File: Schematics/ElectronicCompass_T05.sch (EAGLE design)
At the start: 60 parts, among them Q1 SPB80P06P, Q2 SPB80P06P, Q3 SPB80P06P, Q4 SPB80P06P, U1 ATMEGA32U4, X1 USBSMD

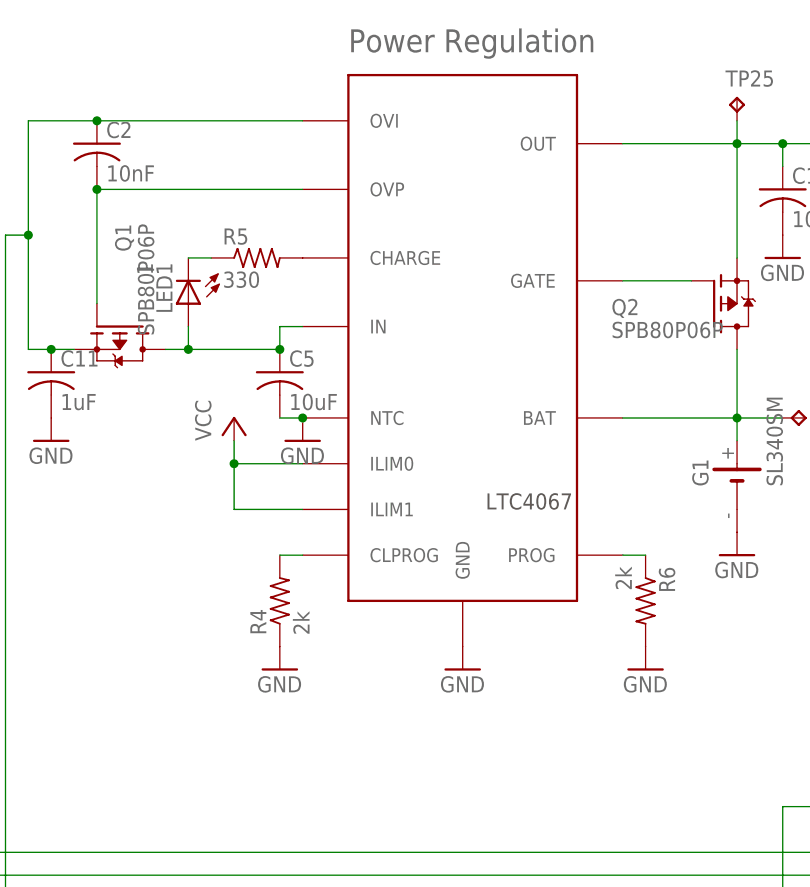
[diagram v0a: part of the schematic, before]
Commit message: board layout continued
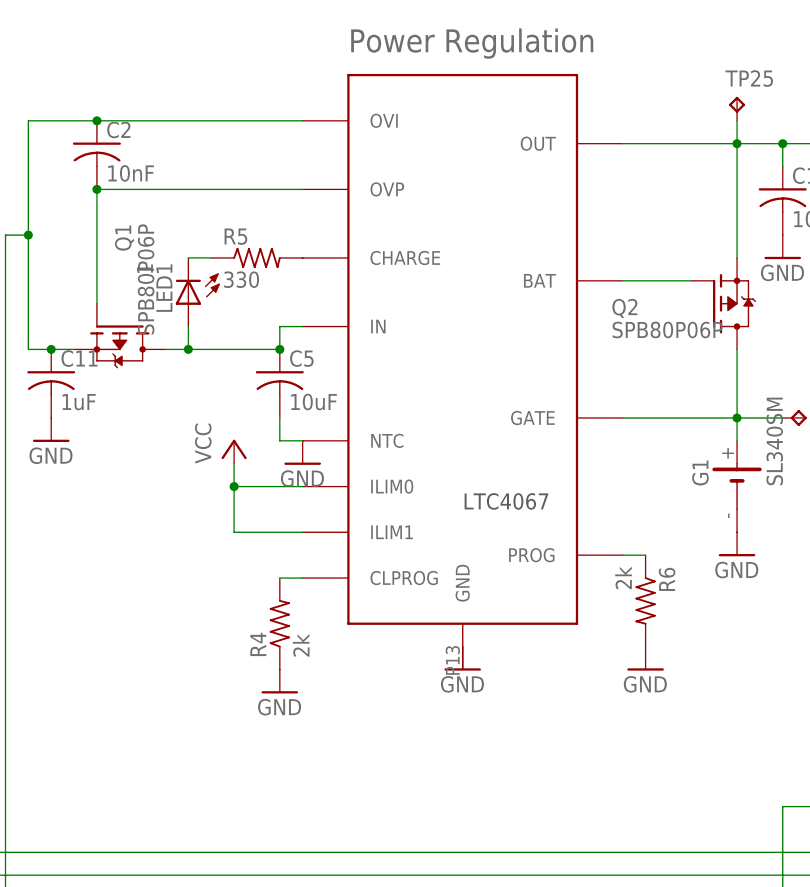
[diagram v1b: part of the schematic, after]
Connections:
- net GND: no longer U$1.GND, U$1.NTC
- net N$16: now also U$1.BAT; no longer U$1.GATE
- net N$4: no longer U$1.CLPROG
- net N$5: now also U$1.GATE; no longer U$1.BAT
- net VCC: no longer U$1.ILIM0, U$1.ILIM1
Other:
- moved on the sheet: R4
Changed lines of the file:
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@@
 <part name="GND14" library="supply1" deviceset="GND" device=""/>
 <part name="C2" library="rcl" deviceset="C-US" device="C0805" value="10nF"/>
-<part name="U$1" library="LTC4067" deviceset="LTC4067" device=""/>
 <part name="C3" library="rcl" deviceset="C-US" device="C0805" value="0.1uF"/>
 <part name="TP26" library="testpad" deviceset="TP" device="TP06R"/>
 <part name="TP27" library="testpad" deviceset="TP" device="TP06R"/>
 <part name="TP28" library="testpad" deviceset="TP" device="TP06R"/>
+<part name="U$1" library="LTC4067" deviceset="LTC4067" device=""/>
 </parts>
 <sheets>
@@
 <frame x1="-25.4" y1="-121.92" x2="276.86" y2="88.9" columns="8" rows="5" layer="97"/>
 <text x="243.84" y="-40.64" size="1.778" layer="97">LCD Mounting/TP</text>
-<text x="53.34" y="27.94" size="1.778" layer="97">LTC4067</text>
+<text x="50.8" y="27.94" size="1.778" layer="97">LTC4067</text>
 <text x="210.82" y="10.16" size="1.778" layer="97">LSM303DLM</text>
 <text x="213.36" y="-66.04" size="1.778" layer="97">Nokia 5110</text>
@@
 <instance part="JP6" gate="G$1" x="175.26" y="-86.36"/>
 <instance part="JP7" gate="G$1" x="182.88" y="-86.36"/>
-<instance part="R4" gate="G$1" x="30.48" y="17.78" rot="R90"/>
+<instance part="R4" gate="G$1" x="30.48" y="15.24" rot="R90"/>
 <instance part="R5" gate="G$1" x="27.94" y="55.88"/>
 <instance part="R6" gate="G$1" x="71.12" y="17.78" rot="R270"/>
@@
 <instance part="GND9" gate="1" x="50.8" y="10.16"/>
 <instance part="GND15" gate="1" x="71.12" y="10.16"/>
-<instance part="GND16" gate="1" x="30.48" y="10.16"/>
-<instance part="P+5" gate="VCC" x="25.4" y="38.1"/>
+<instance part="GND16" gate="1" x="30.48" y="7.62"/>
+<instance part="P+5" gate="VCC" x="25.4" y="35.56"/>
 <instance part="LED1" gate="G$1" x="20.32" y="50.8" rot="R180"/>
 <instance part="Q1" gate="G$1" x="12.7" y="48.26" rot="MR270"/>
@@
 <instance part="C12" gate="G$1" x="76.2" y="-17.78"/>
 <instance part="GND17" gate="1" x="76.2" y="-25.4"/>
-<instance part="GND18" gate="1" x="33.02" y="35.56"/>
+<instance part="GND18" gate="1" x="33.02" y="33.02"/>
 <instance part="G1" gate="G$1" x="81.28" y="30.48" rot="R90"/>
 <instance part="GND19" gate="1" x="81.28" y="22.86"/>
@@
 <instance part="GND14" gate="1" x="5.08" y="35.56"/>
 <instance part="C2" gate="G$1" x="10.16" y="68.58"/>
-<instance part="U$1" gate="G$1" x="50.8" y="40.64" rot="R270"/>
 <instance part="C3" gate="G$1" x="121.92" y="7.62"/>
 <instance part="TP26" gate="G$1" x="180.34" y="-33.02" rot="R270"/>
 <instance part="TP27" gate="G$1" x="180.34" y="-48.26" rot="R270"/>
 <instance part="TP28" gate="G$1" x="180.34" y="-43.18" rot="R270"/>
+<instance part="U$1" gate="G$1" x="50.8" y="45.72" rot="R270"/>
 </instances>
 <busses>
@@
 <pinref part="GND18" gate="1" pin="GND"/>
 <pinref part="C5" gate="G$1" pin="2"/>
-<wire x1="30.48" y1="38.1" x2="33.02" y2="38.1" width="0.1524" layer="91"/>
-<pinref part="U$1" gate="G$1" pin="NTC"/>
-<junction x="33.02" y="38.1"/>
+<wire x1="30.48" y1="38.1" x2="30.48" y2="35.56" width="0.1524" layer="91"/>
+<wire x1="30.48" y1="35.56" x2="33.02" y2="35.56" width="0.1524" layer="91"/>
 </segment>
 <segment>
 <pinref part="C11" gate="G$1" pin="2"/>
 <pinref part="GND14" gate="1" pin="GND"/>
-</segment>
-<segment>
-<pinref part="GND9" gate="1" pin="GND"/>
-<pinref part="U$1" gate="G$1" pin="GND"/>
 </segment>
 <segment>
@@
 </segment>
 <segment>
-<wire x1="33.02" y1="27.94" x2="25.4" y2="27.94" width="0.1524" layer="91"/>
+<wire x1="33.02" y1="25.4" x2="25.4" y2="25.4" width="0.1524" layer="91"/>
 <pinref part="P+5" gate="VCC" pin="VCC"/>
-<wire x1="25.4" y1="27.94" x2="25.4" y2="33.02" width="0.1524" layer="91"/>
-<wire x1="25.4" y1="33.02" x2="25.4" y2="35.56" width="0.1524" layer="91"/>
-<wire x1="33.02" y1="33.02" x2="25.4" y2="33.02" width="0.1524" layer="91"/>
-<junction x="25.4" y="33.02"/>
-<pinref part="U$1" gate="G$1" pin="ILIM0"/>
-<pinref part="U$1" gate="G$1" pin="ILIM1"/>
+<wire x1="25.4" y1="25.4" x2="25.4" y2="30.48" width="0.1524" layer="91"/>
+<wire x1="25.4" y1="30.48" x2="25.4" y2="33.02" width="0.1524" layer="91"/>
+<wire x1="33.02" y1="30.48" x2="25.4" y2="30.48" width="0.1524" layer="91"/>
+<junction x="25.4" y="30.48"/>
 </segment>
 </net>
@@
 <segment>
 <pinref part="R4" gate="G$1" pin="2"/>
-<wire x1="30.48" y1="22.86" x2="33.02" y2="22.86" width="0.1524" layer="91"/>
-<pinref part="U$1" gate="G$1" pin="CLPROG"/>
+<wire x1="30.48" y1="20.32" x2="33.02" y2="20.32" width="0.1524" layer="91"/>
 </segment>
 </net>
@@
 <wire x1="81.28" y1="38.1" x2="81.28" y2="45.72" width="0.1524" layer="91"/>
 <junction x="81.28" y="38.1"/>
-<pinref part="U$1" gate="G$1" pin="BAT"/>
+<pinref part="U$1" gate="G$1" pin="GATE"/>
 </segment>
 </net>
@@
 <pinref part="Q2" gate="G$1" pin="G"/>
 <wire x1="68.58" y1="53.34" x2="76.2" y2="53.34" width="0.1524" layer="91"/>
-<pinref part="U$1" gate="G$1" pin="GATE"/>
+<pinref part="U$1" gate="G$1" pin="BAT"/>
 </segment>
 </net>
@@
 </segment>
 </net>
-<net name="N$7" class="0">
-<segment>
-<pinref part="R5" gate="G$1" pin="2"/>
-<pinref part="U$1" gate="G$1" pin="CHARGE"/>
-</segment>
-</net>
 <net name="N$37" class="0">
 <segment>
@@
 </segment>
 </net>
+<net name="N$7" class="0">
+<segment>
+<pinref part="R5" gate="G$1" pin="2"/>
+<pinref part="U$1" gate="G$1" pin="CHARGE"/>
+</segment>
+</net>
